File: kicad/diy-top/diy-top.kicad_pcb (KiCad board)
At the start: 2 copper layers, 40 x 34.3 mm, 8 parts, among them J1 Conn_01x15_MountingPin

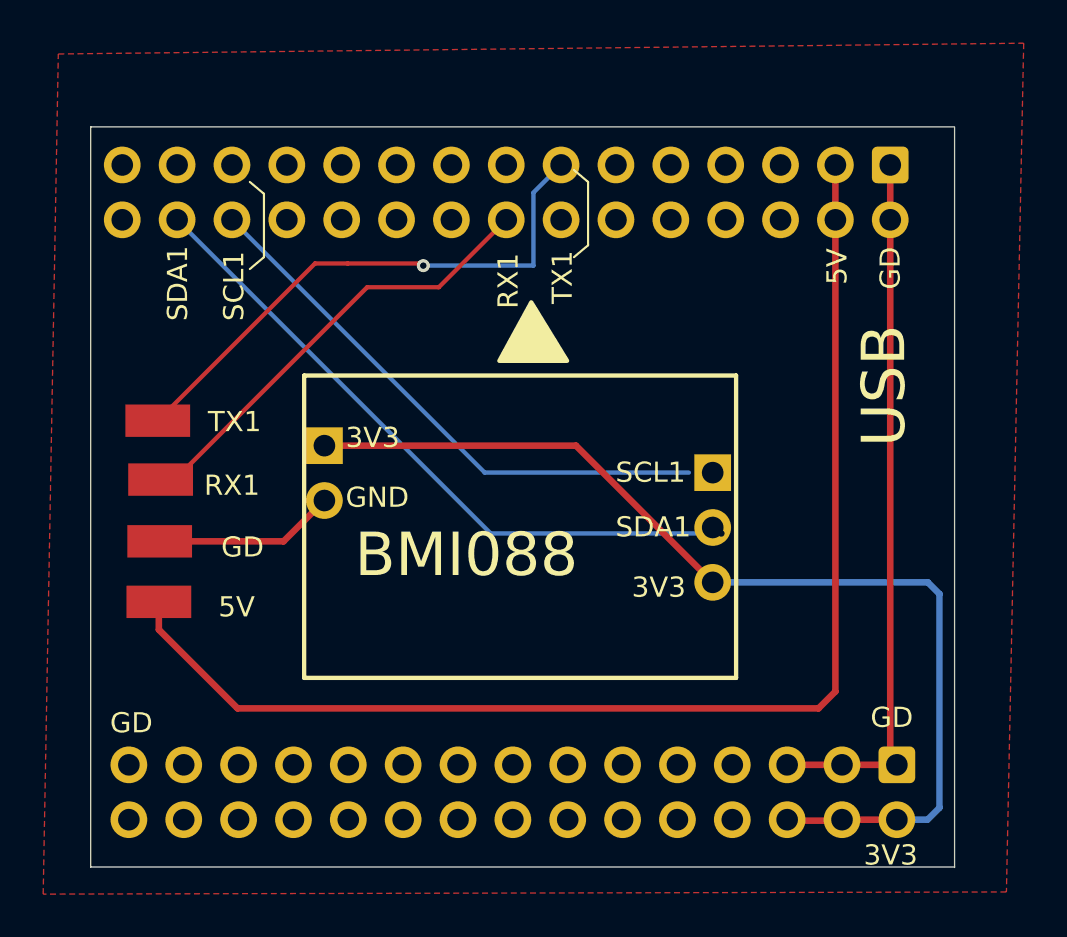
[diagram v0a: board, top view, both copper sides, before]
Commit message: modified:   kicad/diy-top/diy-top.kicad_pcb
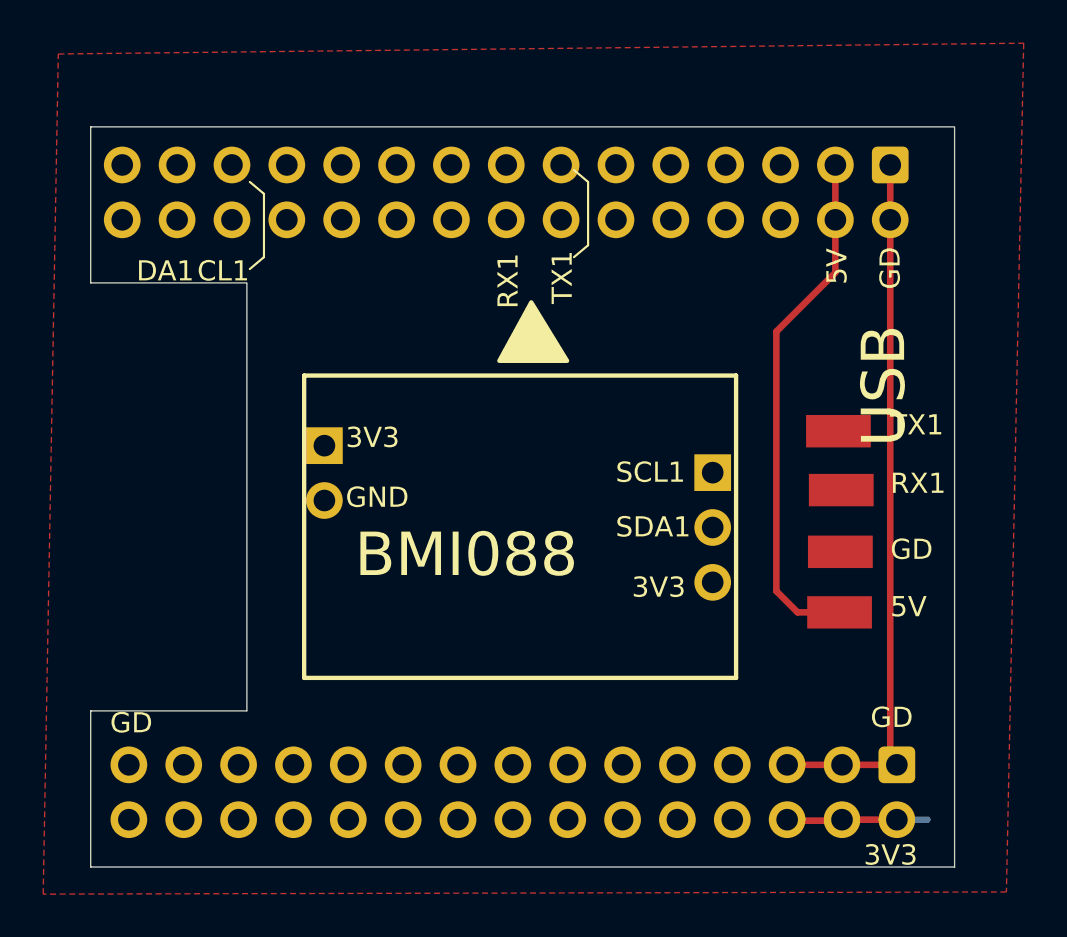
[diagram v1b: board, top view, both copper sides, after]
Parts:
- moved GND_PAD18 31.5 mm to (161.9, 108.5)
- moved GND_PAD19 31.5 mm to (161.8, 110.2)
- moved GND_PAD21 31.5 mm to (161.8, 102.9)
- moved GND_PAD20 31.5 mm to (161.9, 105.6)
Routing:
- net /3V3: track 48.6 -> 6.64 mm
- net /5V: track 58.8 -> 24.2 mm
- net /SDA1: track 31.7 -> 0.12 mm, vias 1 -> 0
- net (no net): track 26.0 -> 0.00 mm
- net /TX1: track 25.6 -> 0.00 mm, vias 1 -> 0
- net /RX1: track 21.0 -> 0.00 mm
- net /GND: track 41.4 -> 33.0 mm
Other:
- outline, holes or cut-outs redrawn
- board text added: "CL1"
- board text added: "DA1"

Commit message: modified:   kicad/diy-bottom/diy-bottom.kicad_pcb
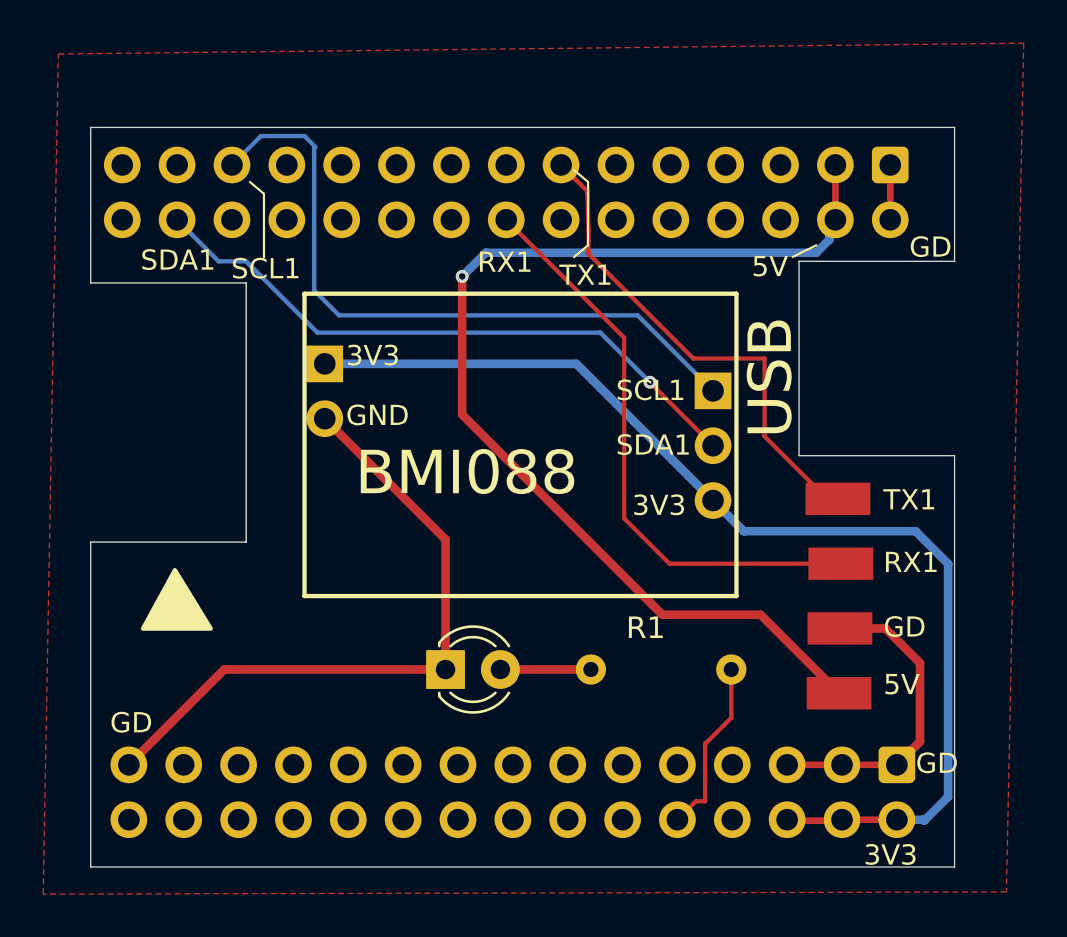
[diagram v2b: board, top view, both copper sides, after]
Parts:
- added D1: LED, LED_THT:LED_D3.0mm, F.Cu at (143.4, 111.9)
- added R1: R, Resistor_THT:R_Axial_DIN0204_L3.6mm_D1.6mm_P5.08mm_Horizontal, F.Cu at (150.2, 111.9)
- moved Motor5 3.79 mm to (155.1, 99.0)
- moved PMW3901_PWR2 3.79 mm to (140.8, 97.7)
- moved GND_PAD18 2.95 mm to (161.9, 111.5)
- moved GND_PAD19 2.95 mm to (161.8, 113.2)
- moved GND_PAD20 2.95 mm to (161.8, 108.6)
- moved GND_PAD21 2.95 mm to (161.8, 105.8)
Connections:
- J1 pad 10: unconnected-(J1-Pin_10-Pad10) -> /PB2
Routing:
- net /3V3: track 6.64 -> 51.6 mm
- net /SCL1: track 0.00 -> 31.6 mm
- net /SDA1: track 0.12 -> 29.3 mm, vias 0 -> 1
- net /RX1: track 0.00 -> 27.0 mm
- net /5V: track 24.2 -> 50.5 mm, vias 0 -> 1
- net /TX1: track 0.00 -> 23.0 mm
- net /GND: track 33.0 -> 47.6 mm
- net /PB2: track 0.00 -> 8.80 mm
- net Net-(D1-A): track 0.00 -> 4.19 mm
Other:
- board size 40 x 34.3 mm -> 40 x 34.2 mm
- board text removed: "CL1"
- board text removed: "DA1"
